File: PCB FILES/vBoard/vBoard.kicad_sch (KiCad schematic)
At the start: 2 parts, among them SW1 SW_Push

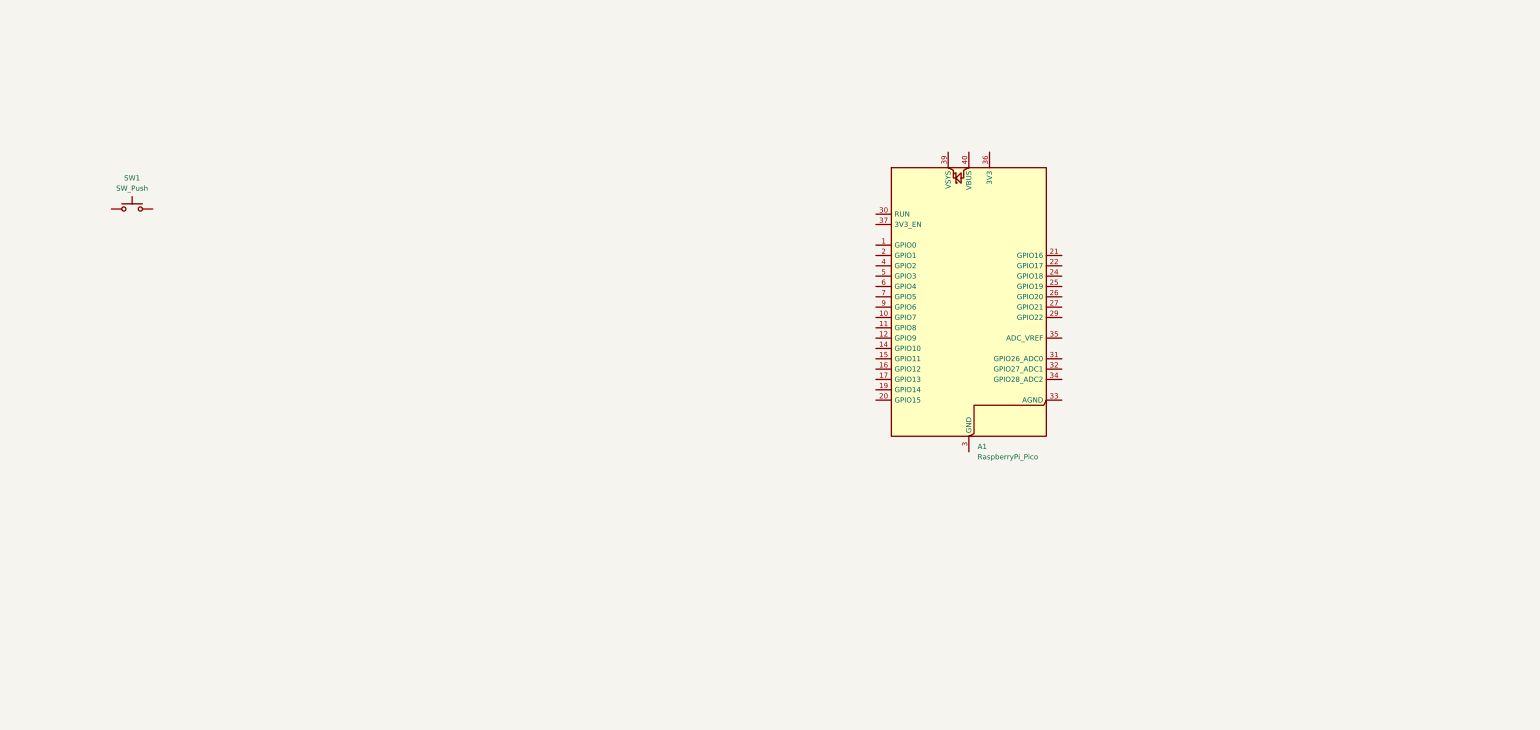
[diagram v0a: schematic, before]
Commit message: ill journal tomorrow
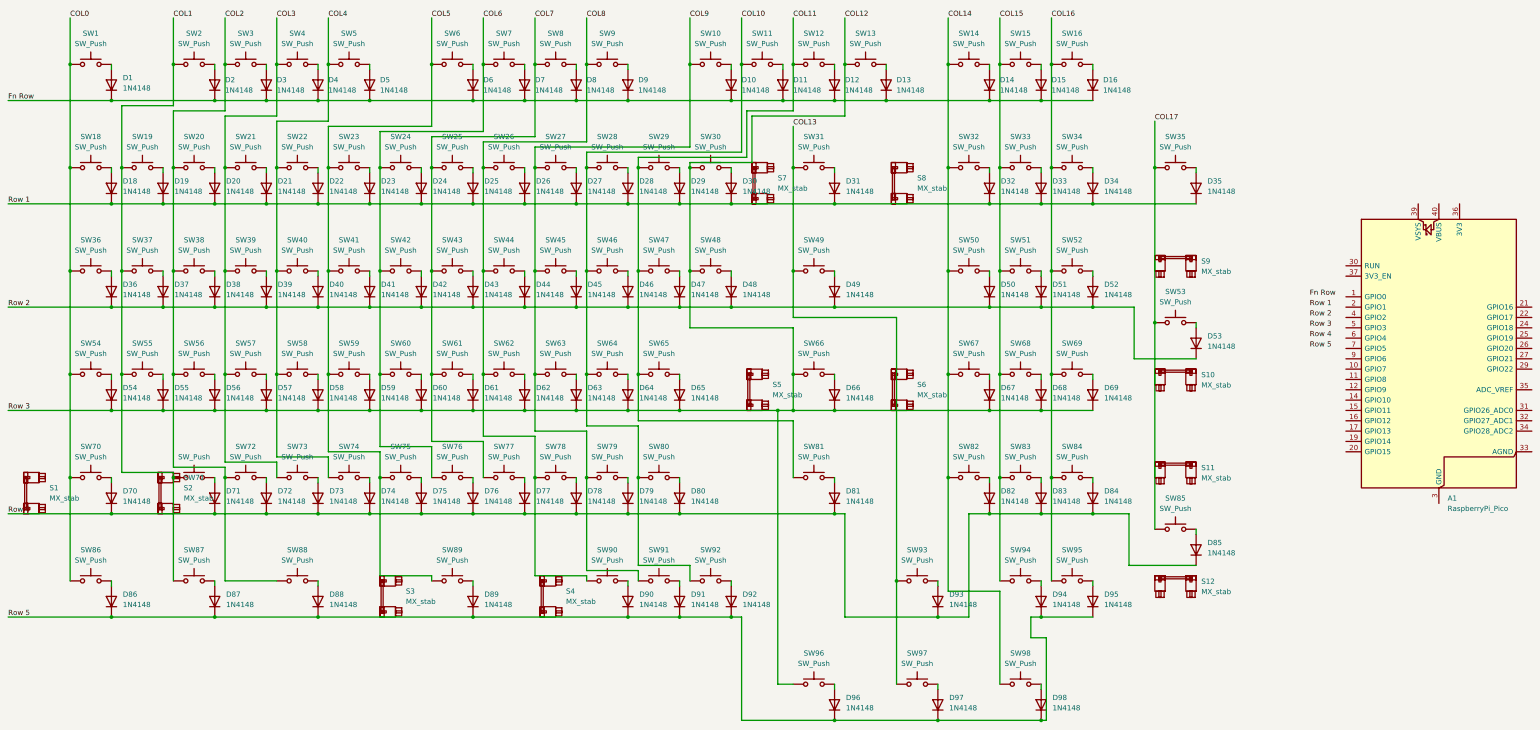
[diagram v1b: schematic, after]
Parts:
- added D1, D10, D11, D12, D13, D14, D15, D16, D18, D19, D2, D20, D21, D22, D23, D24, D25, D26, D27, D28, D29, D3, D30, D31, D32, D33, D34, D35, D36, D37, D38, D39, D4, D40, D41, D42, D43, D44, D45, D46, D47, D48, D49, D5, D50, D51, D52, D53, D54, D55, D56, D57, D58, D59, D6, D60, D61, D62, D63, D64, D65, D66, D67, D68, D69, D7, D70, D71, D72, D73, D74, D75, D76, D77, D78, D79, D8, D80, D81, D82, D83, D84, D85, D86, D87, D88, D89, D9, D90, D91, D92, D93, D94, D95, D96, D97, D98: 1N4148, Diode_THT:D_DO-35_SOD27_P7.62mm_Horizontal, symbol Diode:1N4148
- added S1, S10, S11, S12, S2, S3, S4, S5, S6, S7, S8, S9: MX_stab, PCM_marbastlib-mx:STAB_MX_P_6.25u, symbol PCM_marbastlib-mx:MX_stab
- added SW10, SW11, SW12, SW13, SW14, SW15, SW16, SW18, SW19, SW2, SW20, SW21, SW22, SW23, SW24, SW25, SW26, SW27, SW28, SW29, SW3, SW30, SW31, SW32, SW33, SW34, SW35, SW36, SW37, SW38, SW39, SW4, SW40, SW41, SW42, SW43, SW44, SW45, SW46, SW47, SW48, SW49, SW5, SW50, SW51, SW52, SW53, SW54, SW55, SW56, SW57, SW58, SW59, SW6, SW60, SW61, SW62, SW63, SW64, SW65, SW66, SW67, SW68, SW69, SW7, SW70, SW71, SW72, SW73, SW74, SW75, SW76, SW77, SW78, SW79, SW8, SW80, SW81, SW82, SW83, SW84, SW85, SW86, SW87, SW88, SW89, SW9, SW90, SW91, SW92, SW93, SW94, SW95, SW96, SW97, SW98: SW_Push, Button_Switch_THT:SW_NKK_GW12LJP, symbol Switch:SW_Push
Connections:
- net COL0: now reaches SW1.1
- net COL0: now also SW18.1, SW36.1, SW54.1, SW70.1, SW86.1
- net at SW1.2: now also D1.2 (A)
- new net: D44.2 (A), SW44.2
- new net: D34.2 (A), SW34.2
- new net: D5.2 (A), SW5.2
- new net: D48.2 (A), SW48.2
- new net: D89.2 (A), SW89.2
- new net: D31.2 (A), SW31.2
- new net: D40.2 (A), SW40.2
- new net: D92.2 (A), SW92.2
- new net: D79.2 (A), SW79.2
- new net: D36.2 (A), SW36.2
- new net: D60.2 (A), SW60.2
- new net: D22.2 (A), SW22.2
- new net: D49.2 (A), SW49.2
- new net: D74.2 (A), SW74.2
- new net: D91.2 (A), SW91.2
- new net: D72.2 (A), SW72.2
- new net: D16.2 (A), SW16.2
- new net: D98.2 (A), SW98.2
- new net: D21.2 (A), SW21.2
- new net: D80.2 (A), SW80.2
- new net: D95.2 (A), SW95.2
- new net: D30.2 (A), SW30.2
- new net: D28.2 (A), SW28.2
- new net: D24.2 (A), SW24.2
- new net: D65.2 (A), SW65.2
- new net: D43.2 (A), SW43.2
- new net: D11.2 (A), SW11.2
- new net: D25.2 (A), SW25.2
- new net: D63.2 (A), SW63.2
- new net: D85.2 (A), SW85.2
- new net: D10.2 (A), SW10.2
- new net: D4.2 (A), SW4.2
- new net: D8.2 (A), SW8.2
- new net: D68.2 (A), SW68.2
- new net: D55.2 (A), SW55.2
- new net: D61.2 (A), SW61.2
- new net: D23.2 (A), SW23.2
- new net: D29.2 (A), SW29.2
- new net: D35.2 (A), SW35.2
- new net: D39.2 (A), SW39.2
- new net: D67.2 (A), SW67.2
- new net: D96.2 (A), SW96.2
- new net: D38.2 (A), SW38.2
- new net: D81.2 (A), SW81.2
- new net: D77.2 (A), SW77.2
- new net: D73.2 (A), SW73.2
- new net: D6.2 (A), SW6.2
- new net: D9.2 (A), SW9.2
- new net: D86.2 (A), SW86.2
- new net: D87.2 (A), SW87.2
- new net: D47.2 (A), SW47.2
- new net: D52.2 (A), SW52.2
- new net: D14.2 (A), SW14.2
- new net: D64.2 (A), SW64.2
- new net: D46.2 (A), SW46.2
- new net: D57.2 (A), SW57.2
- new net: D37.2 (A), SW37.2
- new net: D78.2 (A), SW78.2
- new net: D27.2 (A), SW27.2
- new net: D71.2 (A), SW71.2
- new net: D69.2 (A), SW69.2
- new net: D82.2 (A), SW82.2
- new net: D90.2 (A), SW90.2
- new net: D20.2 (A), SW20.2
- new net: D19.2 (A), SW19.2
- new net: D54.2 (A), SW54.2
- new net: D26.2 (A), SW26.2
- new net: D56.2 (A), SW56.2
- new net: D7.2 (A), SW7.2
- new net: D70.2 (A), SW70.2
- new net: D66.2 (A), SW66.2
- new net: D84.2 (A), SW84.2
- new net: D58.2 (A), SW58.2
- new net: D2.2 (A), SW2.2
- new net: D33.2 (A), SW33.2
- new net: D59.2 (A), SW59.2
- new net: D45.2 (A), SW45.2
- new net: D75.2 (A), SW75.2
- new net: D18.2 (A), SW18.2
- new net: D42.2 (A), SW42.2
- new net: D93.2 (A), SW93.2
- new net: D53.2 (A), SW53.2
- new net: D76.2 (A), SW76.2
- new net: D51.2 (A), SW51.2
- new net: D3.2 (A), SW3.2
- new net: D32.2 (A), SW32.2
- new net: D83.2 (A), SW83.2
- new net: D50.2 (A), SW50.2
- new net: D62.2 (A), SW62.2
- new net: D12.2 (A), SW12.2
- new net: D97.2 (A), SW97.2
- new net: D41.2 (A), SW41.2
- new net: D88.2 (A), SW88.2
- new net: D94.2 (A), SW94.2
- new net: D13.2 (A), SW13.2
- new net: D15.2 (A), SW15.2
- new net COL1: SW19.1, SW2.1, SW37.1, SW55.1, SW71.1, SW87.1
- new net COL10: SW11.1, SW28.1, SW46.1, SW64.1, SW80.1, SW92.1
- new net COL11: SW12.1, SW29.1, SW47.1, SW65.1, SW81.1
- new net COL12: D54.1 (K), D55.1 (K), D56.1 (K), D57.1 (K), D58.1 (K), D59.1 (K), D60.1 (K), D61.1 (K), D62.1 (K), D63.1 (K), D64.1 (K), D65.1 (K), D66.1 (K), D67.1 (K), D68.1 (K), D69.1 (K), SW13.1, SW30.1, SW48.1, SW66.1, SW96.1
- new net COL13: SW31.1, SW49.1, SW93.1, SW97.1
- new net COL14: SW14.1, SW32.1, SW50.1, SW67.1, SW82.1, SW98.1
- new net COL15: SW15.1, SW33.1, SW51.1, SW68.1, SW83.1, SW94.1
- new net COL16: SW16.1, SW34.1, SW52.1, SW69.1, SW84.1, SW95.1
- new net COL17: SW35.1, SW53.1, SW85.1
- new net COL2: SW20.1, SW3.1, SW38.1, SW56.1, SW72.1, SW88.1
- new net COL3: SW21.1, SW39.1, SW4.1, SW57.1, SW73.1
- new net COL4: SW22.1, SW40.1, SW5.1, SW58.1, SW74.1
- new net COL5: SW23.1, SW41.1, SW59.1, SW6.1, SW75.1, SW89.1
- new net COL6: SW24.1, SW42.1, SW60.1, SW7.1, SW76.1
- new net COL7: SW25.1, SW43.1, SW61.1, SW77.1, SW8.1
- new net COL8: SW26.1, SW44.1, SW62.1, SW78.1, SW9.1, SW90.1
- new net COL9: SW10.1, SW27.1, SW45.1, SW63.1, SW79.1, SW91.1
- new net Fn Row: D1.1 (K), D10.1 (K), D11.1 (K), D12.1 (K), D13.1 (K), D14.1 (K), D15.1 (K), D16.1 (K), D2.1 (K), D3.1 (K), D4.1 (K), D5.1 (K), D6.1 (K), D7.1 (K), D8.1 (K), D9.1 (K)
- new net Row 1: D18.1 (K), D19.1 (K), D20.1 (K), D21.1 (K), D22.1 (K), D23.1 (K), D24.1 (K), D25.1 (K), D26.1 (K), D27.1 (K), D28.1 (K), D29.1 (K), D30.1 (K), D31.1 (K), D32.1 (K), D33.1 (K), D34.1 (K), D35.1 (K)
- new net Row 2: D36.1 (K), D37.1 (K), D38.1 (K), D39.1 (K), D40.1 (K), D41.1 (K), D42.1 (K), D43.1 (K), D44.1 (K), D45.1 (K), D46.1 (K), D47.1 (K), D48.1 (K), D49.1 (K), D50.1 (K), D51.1 (K), D52.1 (K), D53.1 (K)
- new net Row 4: D70.1 (K), D71.1 (K), D72.1 (K), D73.1 (K), D74.1 (K), D75.1 (K), D76.1 (K), D77.1 (K), D78.1 (K), D79.1 (K), D80.1 (K), D81.1 (K), D82.1 (K), D83.1 (K), D84.1 (K), D85.1 (K), D93.1 (K)
- new net Row 5: D86.1 (K), D87.1 (K), D88.1 (K), D89.1 (K), D90.1 (K), D91.1 (K), D92.1 (K), D94.1 (K), D95.1 (K), D96.1 (K), D97.1 (K), D98.1 (K)
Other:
- moved on the sheet: A1, SW1
